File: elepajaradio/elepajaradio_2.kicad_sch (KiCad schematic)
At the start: 34 parts, among them Q1 2N2219, Q2 2N2219, SW1 RotaryEncoder, U1 ATmega328P-A, U2 OLED_I2C, U3 Opamp_Dual, Y1 Crystal

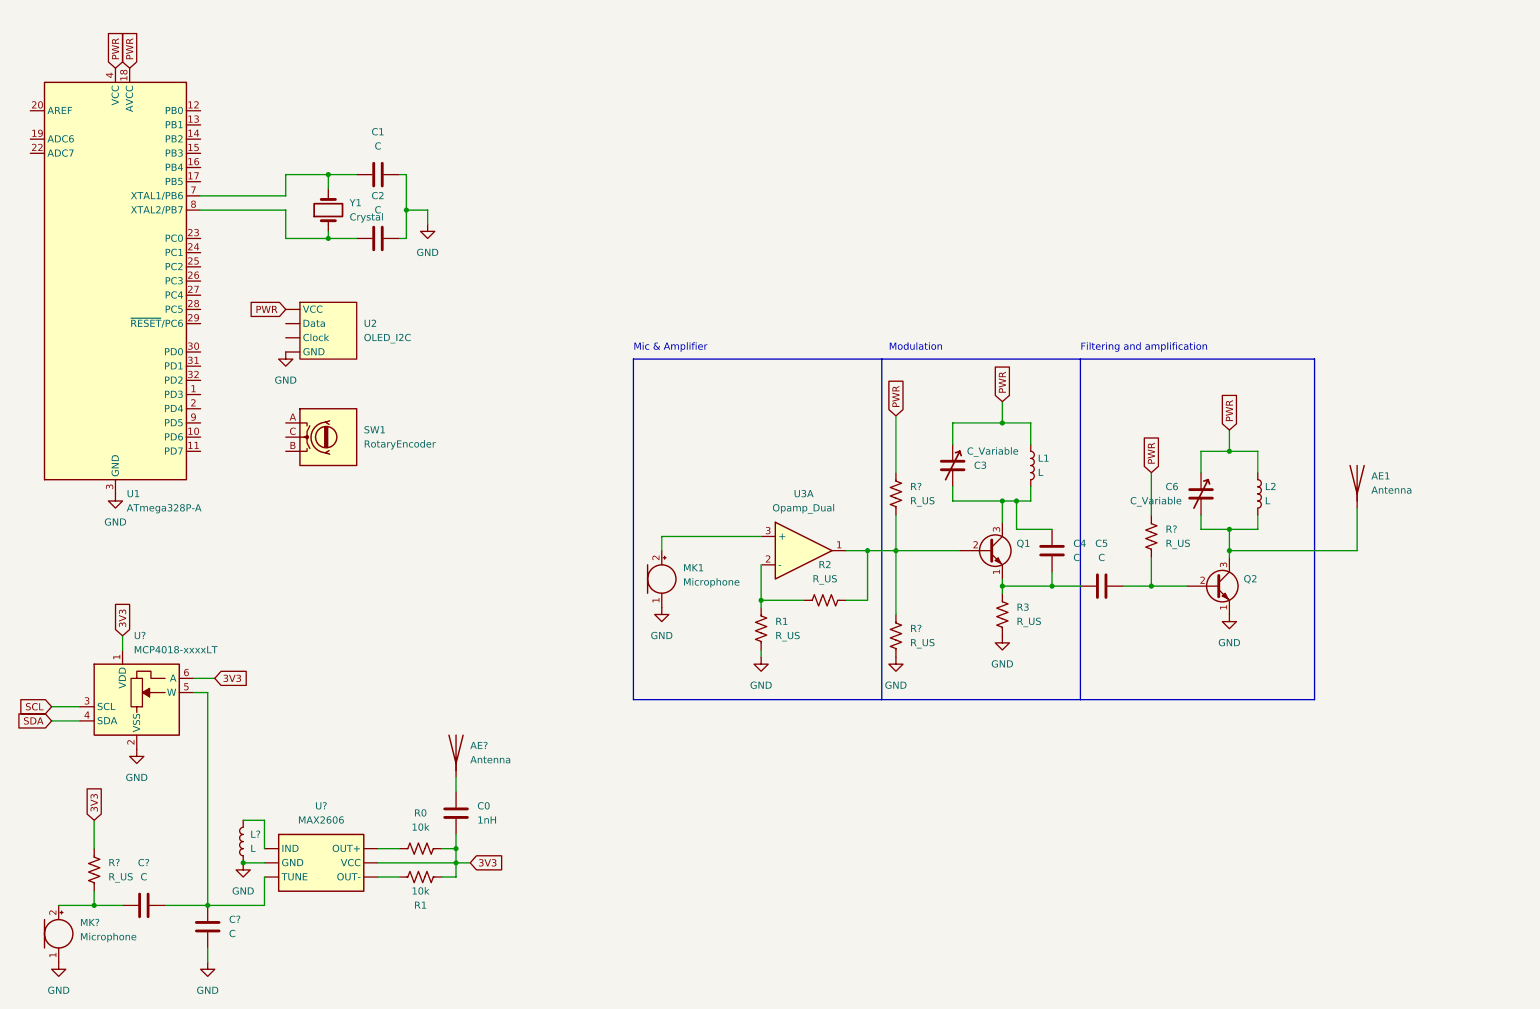
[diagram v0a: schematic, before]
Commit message: 2
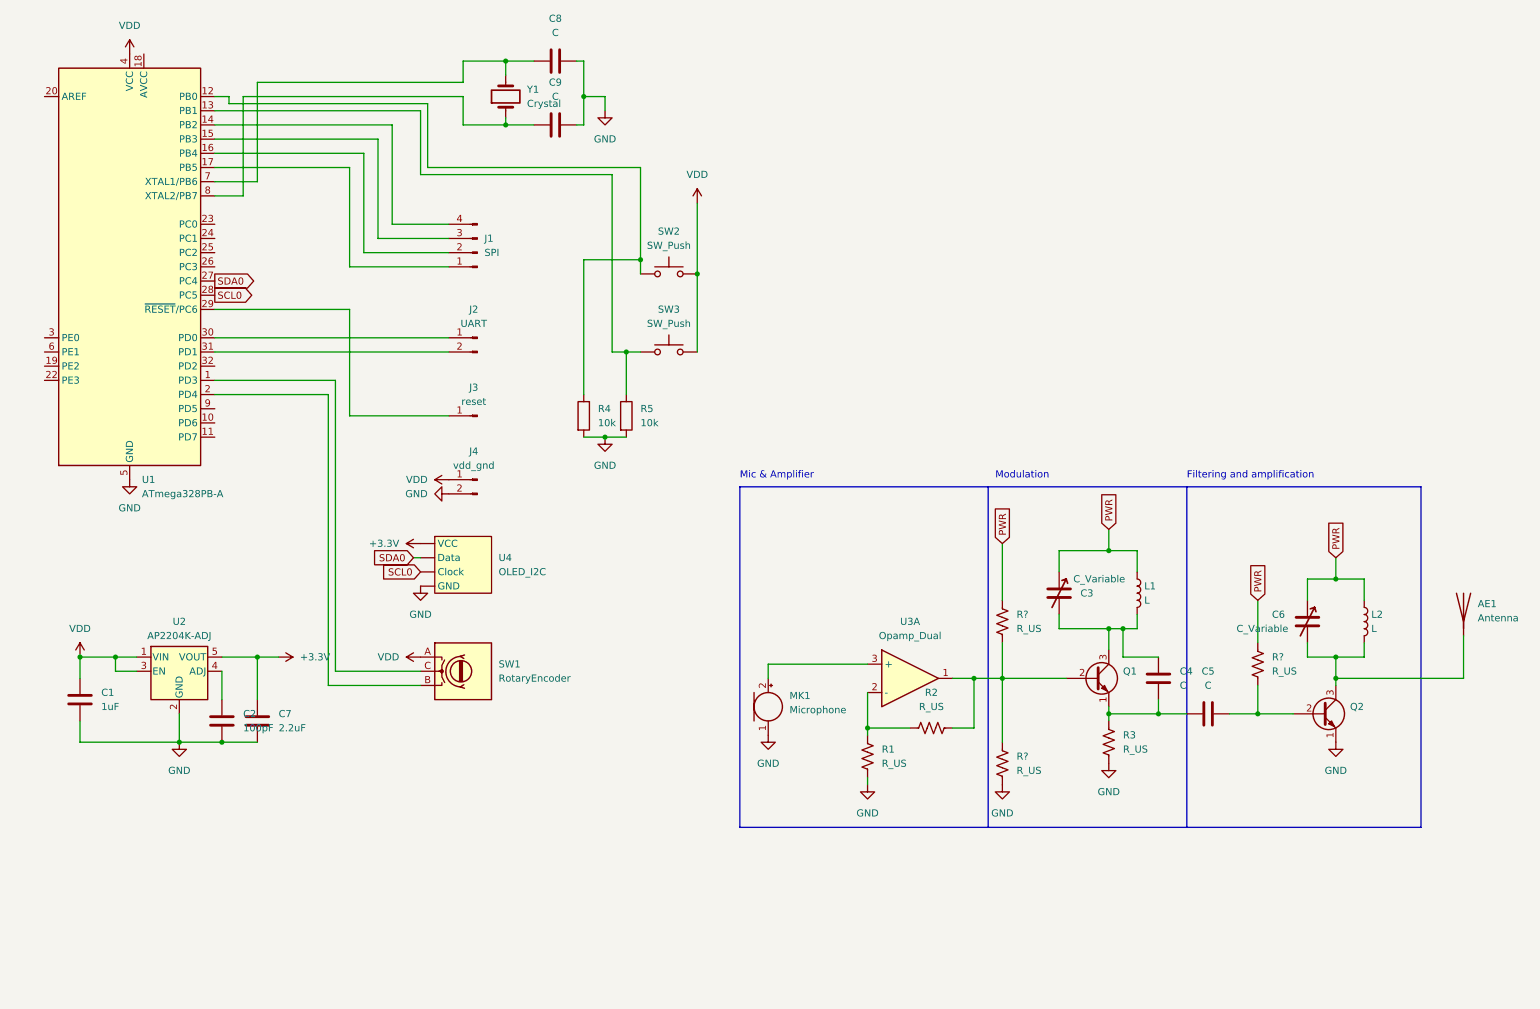
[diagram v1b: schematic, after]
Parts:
- removed AE?: Antenna, symbol Device:Antenna
- removed C0: 1nH, symbol Device:C
- removed C? (x2): C, symbol Device:C
- removed L?: L, symbol Device:L
- removed MK?: Microphone, symbol Device:Microphone
- removed R0, R1: 10k, Resistor_SMD:R_0201_0603Metric_Pad0.64x0.40mm_HandSolder, symbol Device:R_US
- removed R?: R_US, symbol Device:R_US
- removed U1: ATmega328P-A, Package_QFP:TQFP-32_7x7mm_P0.8mm, symbol MCU_Microchip_ATmega:ATmega328P-A
- removed U2: OLED_I2C, symbol oled_lafvin:OLED_I2C
- removed U?: MAX2606, Package_TO_SOT_SMD:SOT-23-6, symbol max2606:MAX2606
- removed U?: MCP4018-xxxxLT, Package_TO_SOT_SMD:SOT-363_SC-70-6, symbol Potentiometer_Digital:MCP4018-xxxxLT
- added C7: 2.2uF, symbol Device:C
- added C8, C9: C, symbol Device:C
- added J1: SPI, symbol Connector:Conn_01x04_Pin
- added J2: UART, symbol Connector:Conn_01x02_Pin
- added J3: reset, symbol Connector:Conn_01x01_Pin
- added J4: vdd_gnd, symbol Connector:Conn_01x02_Pin
- added R4, R5: 10k, symbol Device:R
- added SW2, SW3: SW_Push, symbol Switch:SW_Push
- added U1: ATmega328PB-A, Package_QFP:TQFP-32_7x7mm_P0.8mm, symbol MCU_Microchip_ATmega:ATmega328PB-A
- added U2: AP2204K-ADJ, Package_TO_SOT_SMD:SOT-23-5, symbol Regulator_Linear:AP2204K-ADJ
- added U4: OLED_I2C, symbol oled_lafvin:OLED_I2C
- C1: value C -> 1uF
- C2: value C -> 100pF
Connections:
- net GND: now also C7.2, C8.2, C9.2, J4.2 (Pin_2), R4.2, R5.2, U1.21 (GND), U1.5 (GND), U2.2 (GND), U4. (VCC)
- net at C2.1: now also U2.4 (ADJ); no longer Y1.1
- net at Y1.2: now also C8.1, U1.7 (XTAL1/PB6); no longer C1.1
- net VDD: now reaches SW1.A
- net VDD: now also C1.1, J4.1 (Pin_1), SW2.2, SW3.2, U1.4 (VCC), U2.1 (VIN), U2.3 (EN)
- net at SW1.B: now also U1.2 (PD4)
- net at SW1.C: now also U1.1 (PD3)
- new net: R5.1, SW3.1, U1.13 (PB1)
- new net: J1.1 (Pin_1), U1.17 (PB5)
- new net: J1.2 (Pin_2), U1.16 (PB4)
- new net: J1.3 (Pin_3), U1.15 (PB3)
- new net: J1.4 (Pin_4), U1.14 (PB2)
- new net: C9.1, U1.8 (XTAL2/PB7), Y1.1
- new net: R4.1, SW2.1, U1.12 (PB0)
- new net: J3.1 (Pin_1), U1.29 (~{RESET}/PC6)
- new net: J2.1 (Pin_1), U1.30 (PD0)
- new net: J2.2 (Pin_2), U1.31 (PD1)
- new net +3.3V: C7.1, U2.5 (VOUT), U4. (VCC)
- new net SCL0: U1.28 (PC5), U4. (VCC)
- new net SDA0: U1.27 (PC4), U4. (VCC)
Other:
- moved on the sheet: AE1, C3, C4, C5, C6, L1, L2, MK1, Q1, Q2, R1, R2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
